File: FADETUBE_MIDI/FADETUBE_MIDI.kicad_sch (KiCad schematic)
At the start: 21 parts, among them J1_DECK_A1 B8B-PH-K-S, J2_DECK_B1 B8B-PH-K-S

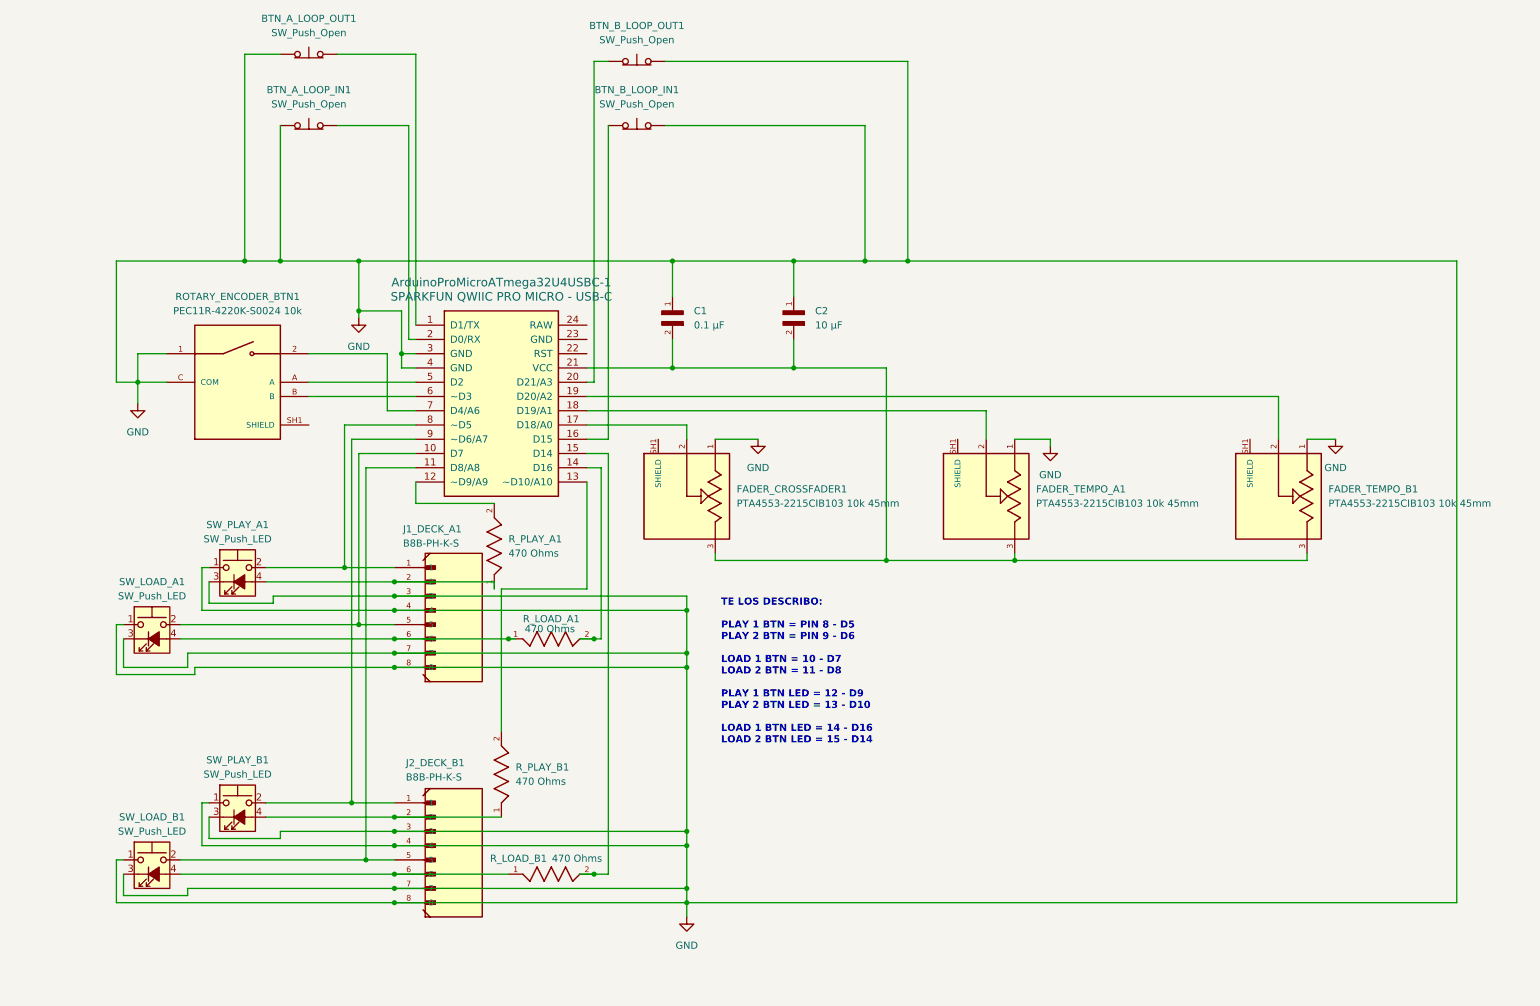
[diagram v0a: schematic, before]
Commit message: new updates
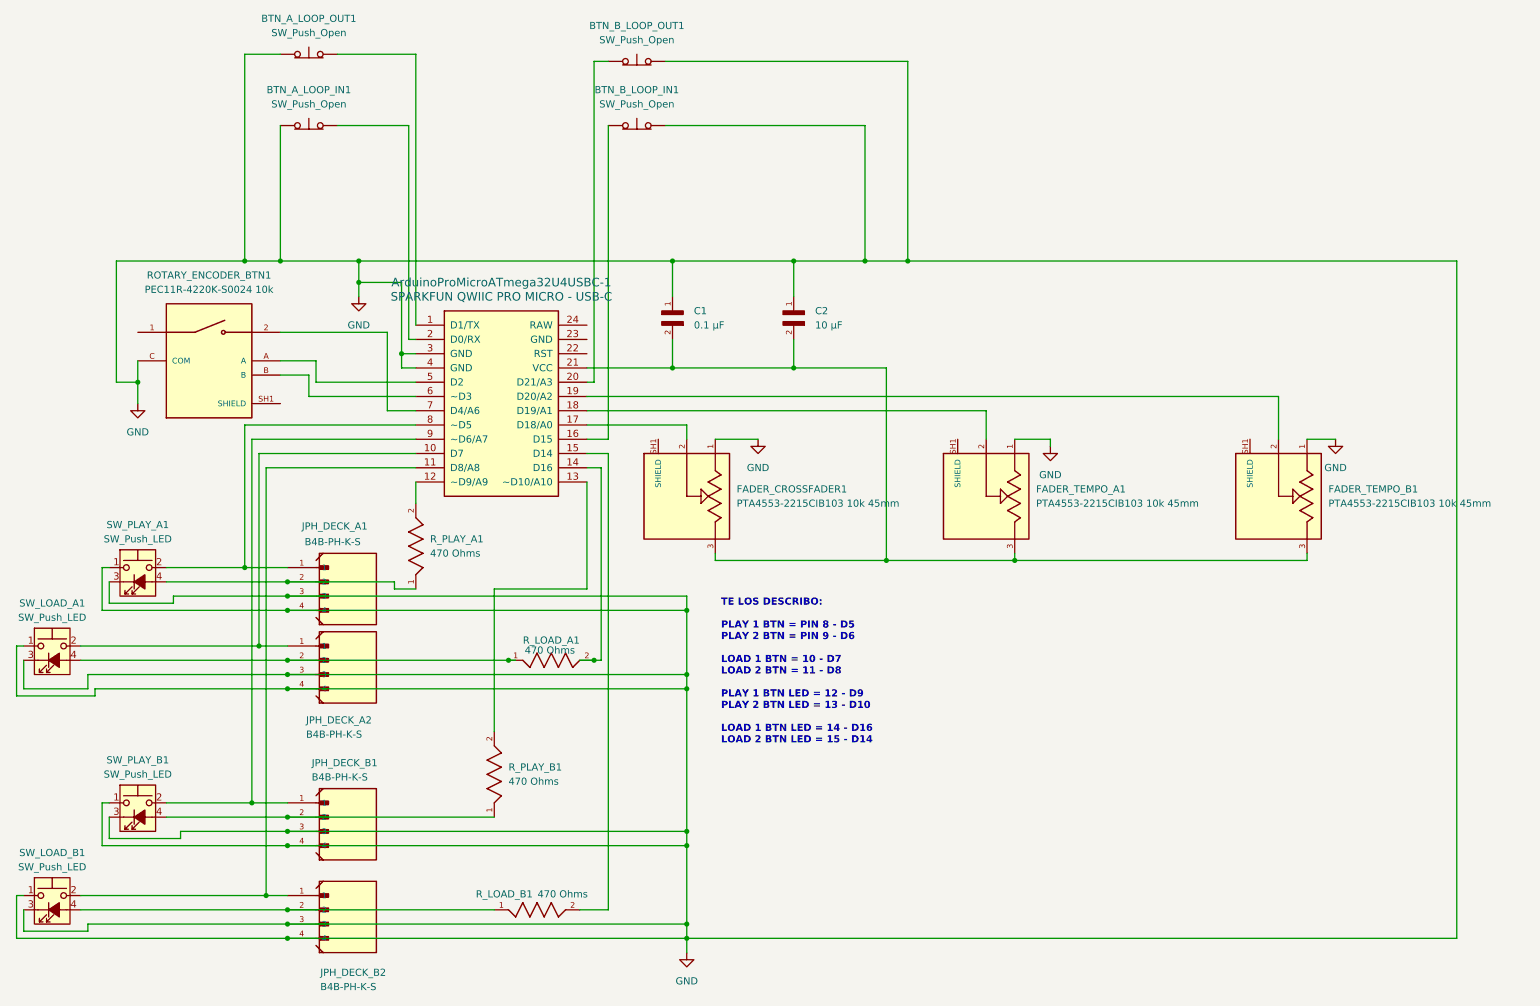
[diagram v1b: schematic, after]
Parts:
- removed J1_DECK_A1, J2_DECK_B1: B8B-PH-K-S, FADETUBE_LIBRARY:JST_B8B-PH-K-S, symbol FADETUBE_LIBRARY:B8B-PH-K-S
- added JPH_DECK_A1, JPH_DECK_A2, JPH_DECK_B1, JPH_DECK_B2: B4B-PH-K-S, FADETUBE_LIBRARY:JST_B4B-PH-K-S, symbol FADETUBE_LIBRARY:B4B-PH-K-S
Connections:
- net GND: now also JPH_DECK_A1.3, JPH_DECK_A1.4, JPH_DECK_A2.3, JPH_DECK_A2.4, JPH_DECK_B1.3, JPH_DECK_B1.4, JPH_DECK_B2.3, JPH_DECK_B2.4; no longer ROTARY_ENCODER_BTN1.1
- net at ArduinoProMicroATmega32U4USBC-1.11 (D8/A8), SW_LOAD_B1.2: now also JPH_DECK_B2.1
- net at R_LOAD_B1.1, SW_LOAD_B1.4 (A): now also JPH_DECK_B2.2
- net at ArduinoProMicroATmega32U4USBC-1.8 (~D5), SW_PLAY_A1.2: now also JPH_DECK_A1.1
- net at R_PLAY_A1.1, SW_PLAY_A1.4 (A): now also JPH_DECK_A1.2
- net at ArduinoProMicroATmega32U4USBC-1.10 (D7), SW_LOAD_A1.2: now also JPH_DECK_A2.1
- net at R_LOAD_A1.1, SW_LOAD_A1.4 (A): now also JPH_DECK_A2.2
- net at ArduinoProMicroATmega32U4USBC-1.9 (~D6/A7), SW_PLAY_B1.2: now also JPH_DECK_B1.1
- net at R_PLAY_B1.1, SW_PLAY_B1.4 (A): now also JPH_DECK_B1.2
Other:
- moved on the sheet: ROTARY_ENCODER_BTN1, R_LOAD_A1, R_LOAD_B1, R_PLAY_A1, R_PLAY_B1, SW_LOAD_A1, SW_LOAD_B1, SW_PLAY_A1, SW_PLAY_B1
